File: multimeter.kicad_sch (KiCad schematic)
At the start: 1 part, among them U1 4543

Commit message: working on decoders
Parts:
- added U10, U7, U8, U9: 4072, symbol 4xxx:4072
- added U2, U3, U4: 4543, symbol 4xxx:4543
- added U5: CC56-12EWA, Display_7Segment:CA56-12EWA, symbol Display_Character:CC56-12EWA
- added U6: 4078, symbol 4xxx_IEEE:4078
- added V1: 5, symbol Simulation_SPICE:VDC
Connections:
- net Qb1: now reaches U1.10 (Qb)
- net Qc1: now reaches U1.11 (Qc)
- net Qd1: now reaches U1.12 (Qd)
- net Qe1: now reaches U1.13 (Qe)
- net Qg1: now reaches U1.14 (Qg)
- net Qf1: now reaches U1.15 (Qf)
- net VDD: now reaches U1.16 (VDD)
- net VDD: now also U2.16 (VDD), U3.16 (VDD), U4.16 (VDD), V1.1
- net GND: now reaches U1.8 (VSS)
- net GND: now also U2.8 (VSS), U3.8 (VSS), U4.8 (VSS), V1.2
- net Qa1: now reaches U1.9 (Qa)
- net Qa1: now also U7.2
- new net Qa2: U2.9 (Qa), U7.3
- new net Qa3: U3.9 (Qa), U7.4
- new net Qa4: U4.9 (Qa), U7.5
- new net Qb2: U2.10 (Qb)
- new net Qb3: U3.10 (Qb)
- new net Qb4: U4.10 (Qb)
- new net Qc2: U2.11 (Qc)
- new net Qc3: U3.11 (Qc)
- new net Qc4: U4.11 (Qc)
- new net Qd2: U2.12 (Qd)
- new net Qd3: U3.12 (Qd)
- new net Qd4: U4.12 (Qd)
- new net Qe2: U2.13 (Qe)
- new net Qe3: U3.13 (Qe)
- new net Qe4: U4.13 (Qe)
- new net Qf2: U2.15 (Qf)
- new net Qf3: U3.15 (Qf)
- new net Qf4: U4.15 (Qf)
- new net Qg2: U2.14 (Qg)
- new net Qg3: U3.14 (Qg)
- new net Qg4: U4.14 (Qg)
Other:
- moved on the sheet: U1

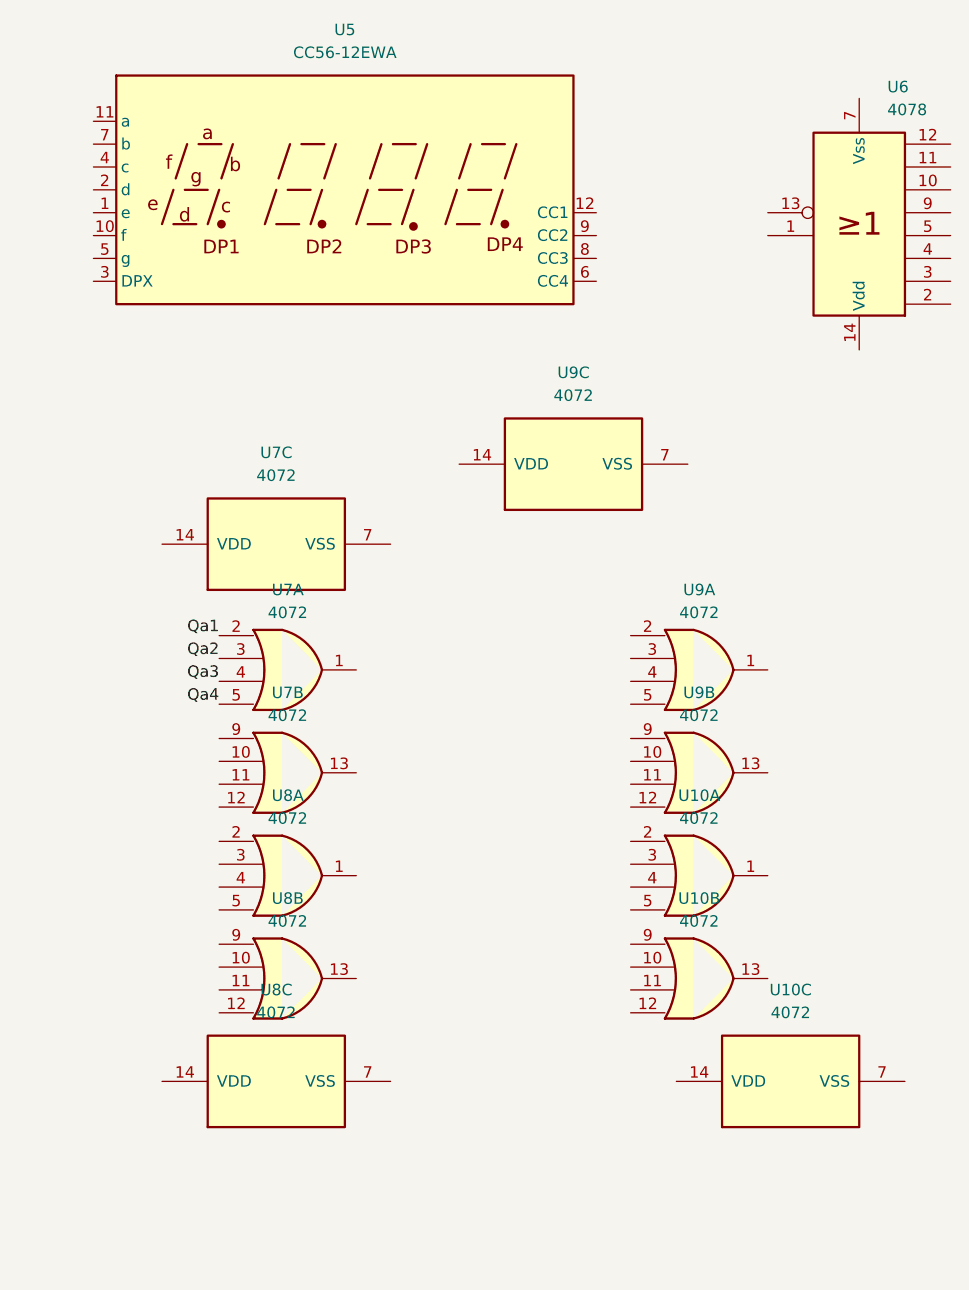
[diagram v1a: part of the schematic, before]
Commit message: multiplexing time
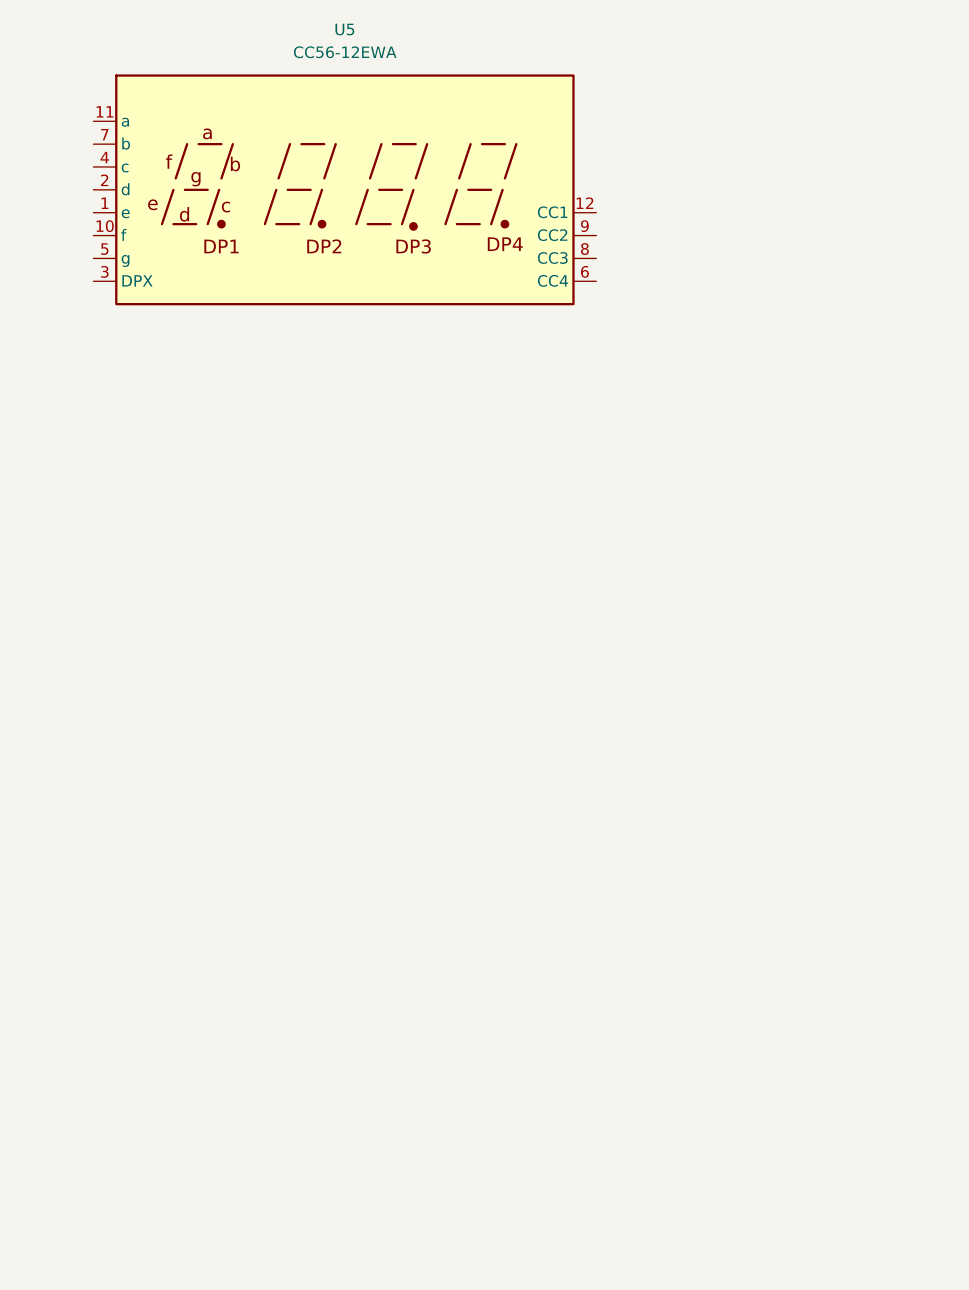
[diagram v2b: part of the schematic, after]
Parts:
- removed U10, U7, U8, U9: 4072, symbol 4xxx:4072
- removed U6: 4078, symbol 4xxx_IEEE:4078
